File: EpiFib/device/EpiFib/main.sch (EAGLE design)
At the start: 6 parts, among them U1 FEATHER_M0, U2 BME280, U3 TFT_TOUCH

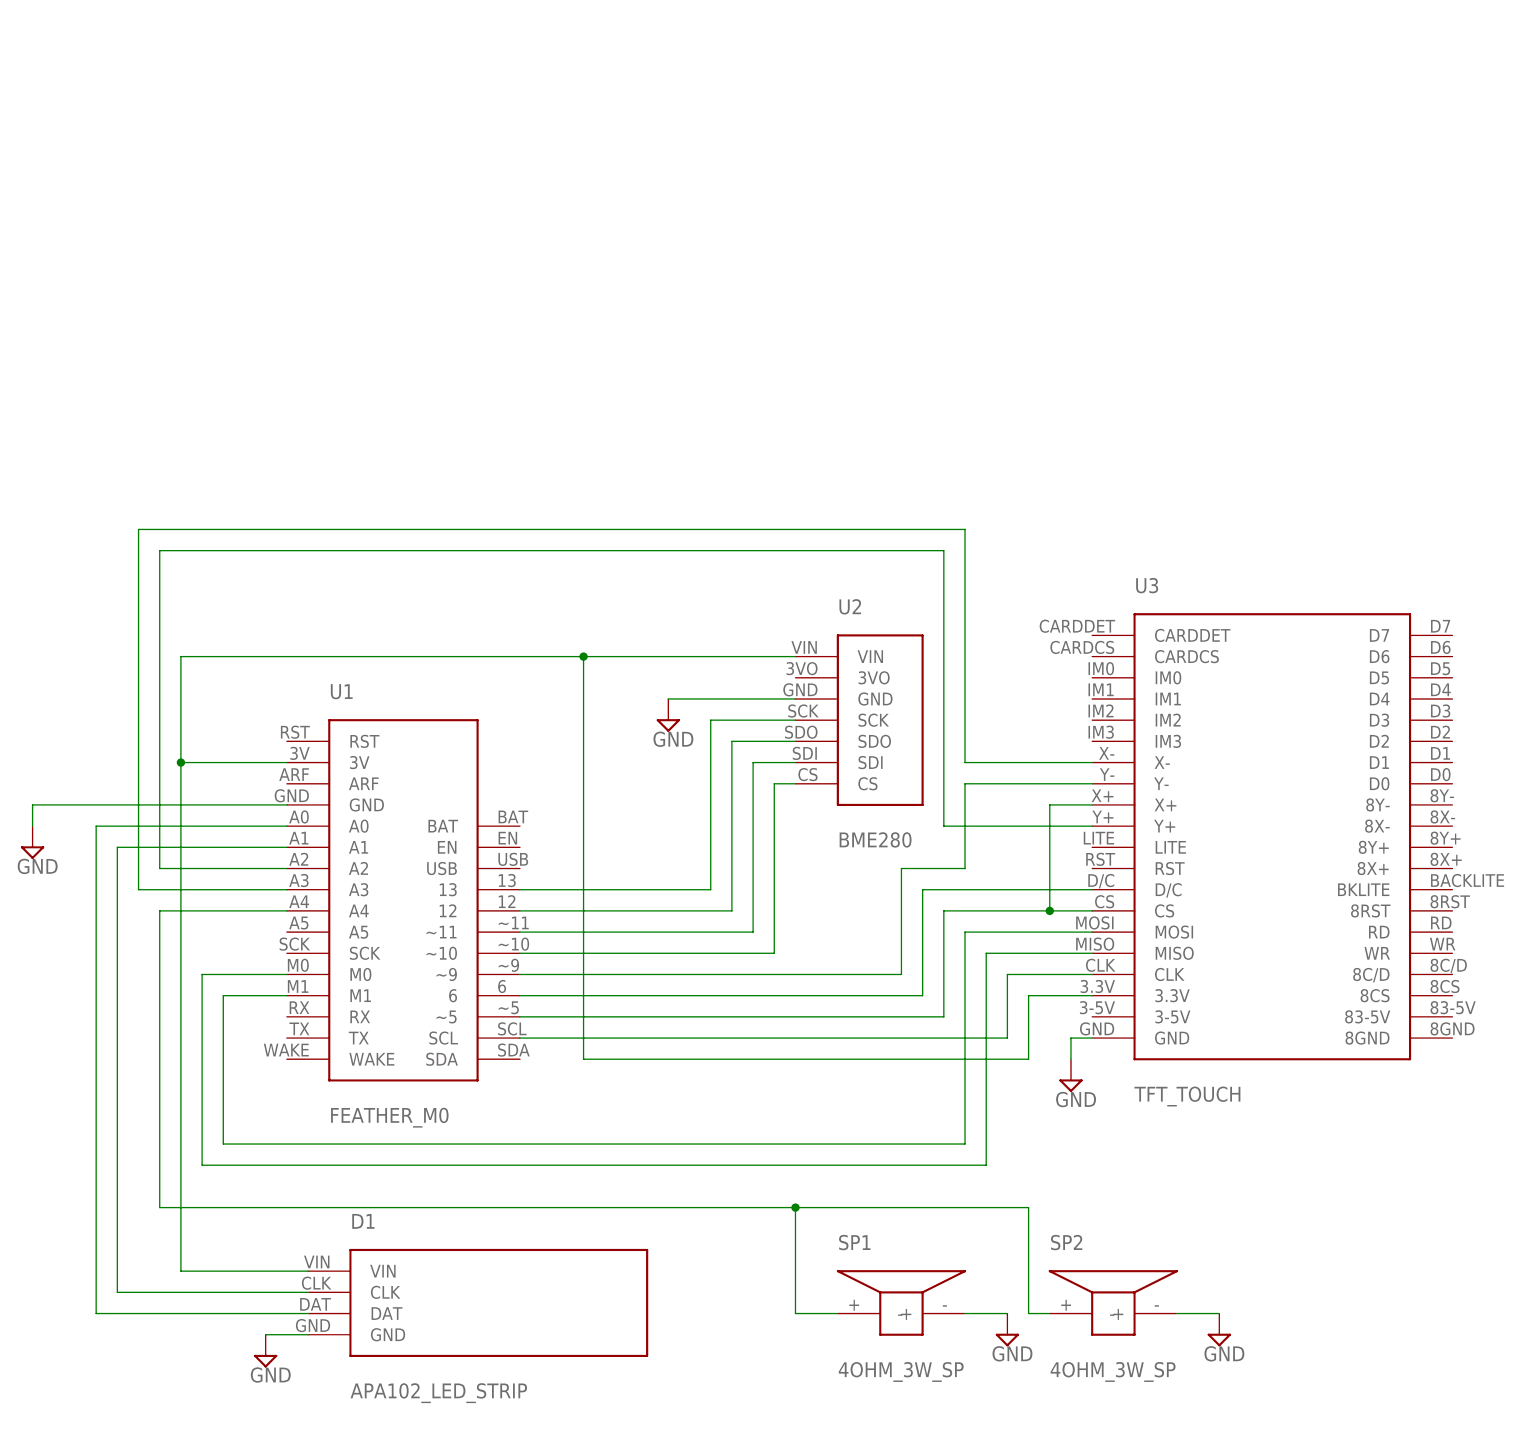
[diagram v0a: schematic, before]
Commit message: final submission
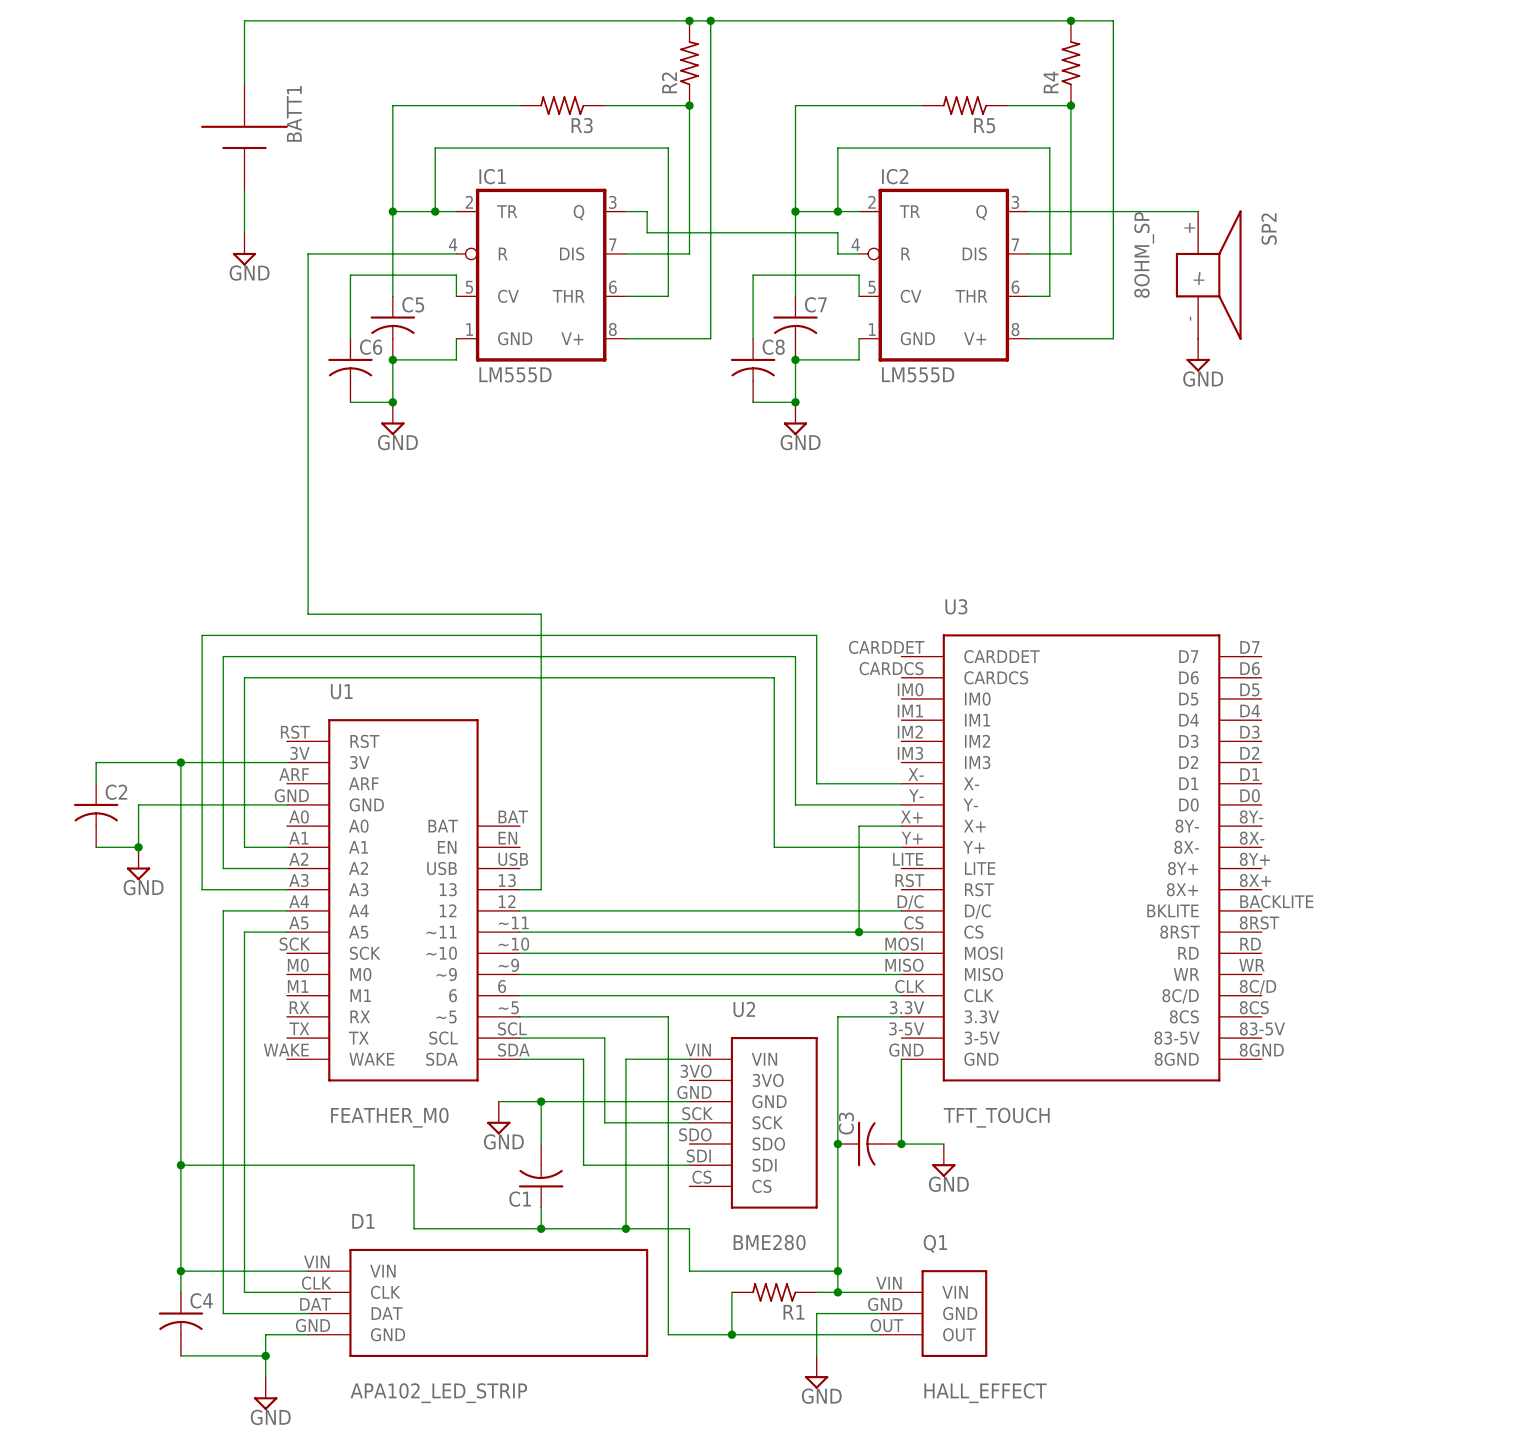
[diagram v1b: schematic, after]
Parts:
- removed SP1: 4OHM_3W_SP, epifib:4OHM_3W_SP
- added BATT1: AAA, adafruit:AAA
- added C1, C2, C3, C4, C5, C6, C7, C8: (no value), rcl:C-US025-024X044
- added IC1, IC2: LM555D, adafruit:LM555D
- added Q1: HALL_EFFECT, epifib:HALL_EFFECT
- added R1, R2, R3, R4, R5: (no value), adafruit:R-US_0207/5V
- SP2: value 4OHM_3W_SP -> 8OHM_SP; device epifib:4OHM_3W_SP -> epifib:8OHM_SP
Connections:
- removed net N$8 (its old number): U1.A2, U3.Y+
- new net N$16: C6.1, IC1.CV
- new net N$18: U1.~9, U3.MISO
- new net N$19: U1.~10, U3.MOSI
- new net N$20: BATT1.-, IC1.V+, IC2.V+, R2.2, R4.2
- new net N$22: IC2.DIS, R4.1, R5.1
- new net N$23: C8.1, IC2.CV
- new net N$24: IC1.Q, IC2.R
- new net N$28: IC1.R, U1.13
- new net N$9: D1.CLK, U1.A5
- net GND: now also BATT1.+, C1.2, C2.2, C3.2, C4.2, C5.2, C6.2, C7.2, C8.2, IC1.GND, IC2.GND, Q1.GND; no longer SP1.-
- net N$1: now also C5.1, IC1.THR, IC1.TR, R3.2; no longer D1.VIN, U1.3V, U2.VIN, U3.3.3V
- net N$10: now also IC2.Q, SP2.+; no longer U1.~9, U3.Y-
- net N$11: now also C1.1, C2.1, C3.1, C4.1, D1.VIN, Q1.VIN, R1.1, U1.3V, U2.VIN, U3.3.3V; no longer D1.CLK, U1.A1
- net N$12: now also Q1.OUT, R1.2, U1.~5; no longer D1.DAT, U1.A0
- net N$13: now also U1.SCL; no longer U1.13
- net N$14: now also U1.SDA; no longer U1.~11
- net N$15: now also IC1.DIS, R2.1, R3.1; no longer U1.12, U2.SDO
- net N$17: now also C7.1, IC2.THR, IC2.TR, R5.2; no longer SP1.+, SP2.+, U1.A4
- net N$2: now also U1.6; no longer U1.SCL
- net N$3: now also U1.A1, U3.Y+; no longer U1.M0, U3.MISO
- net N$4: now also U1.A2, U3.Y-; no longer U1.M1, U3.MOSI
- net N$5: now also U1.~11; no longer U1.~5
- net N$6: now also U1.12; no longer U1.6
- net N$7: now also D1.DAT, U1.A4; no longer U1.~10, U2.CS
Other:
- moved on the sheet: SP2, U2, U3
